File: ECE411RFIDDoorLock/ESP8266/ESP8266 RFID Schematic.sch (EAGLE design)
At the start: 32 parts, among them J4 1050170001, M1 SERVO, Q3 MMBT2222ALT1GOSCT-ND, T1 600mA/40V, T2 600mA/40V, U1 CP2104, U2 AP2112K-3.3TRG1, X1 ESP-12E

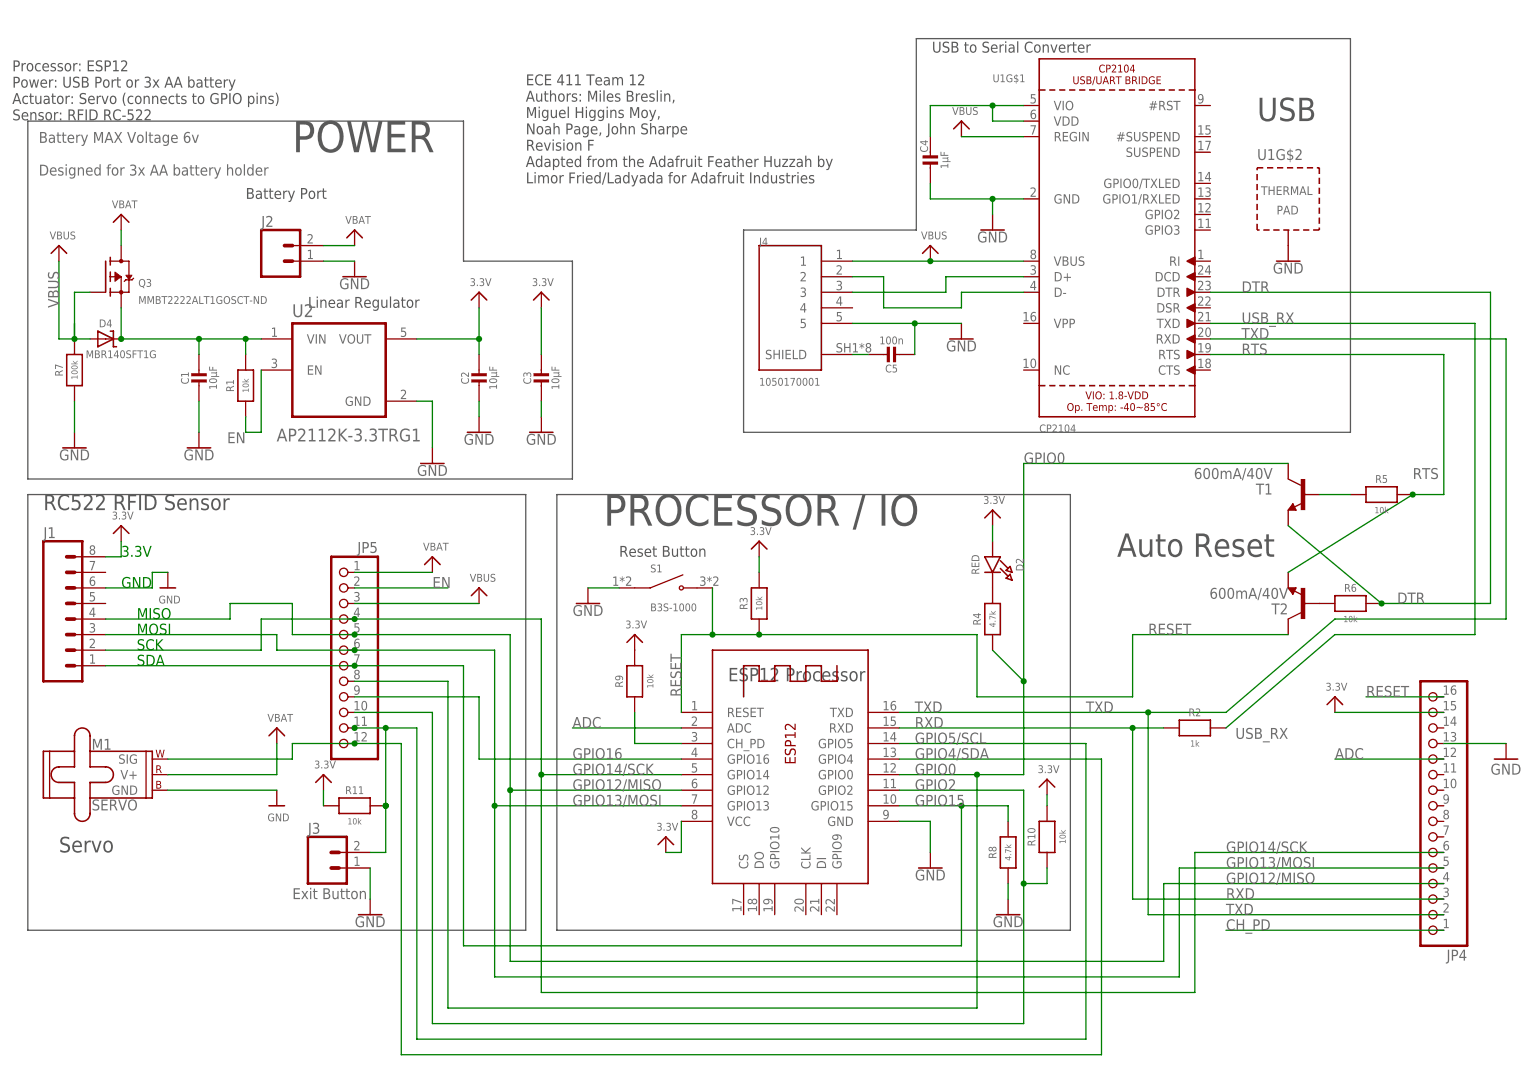
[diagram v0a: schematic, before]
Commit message: Revert
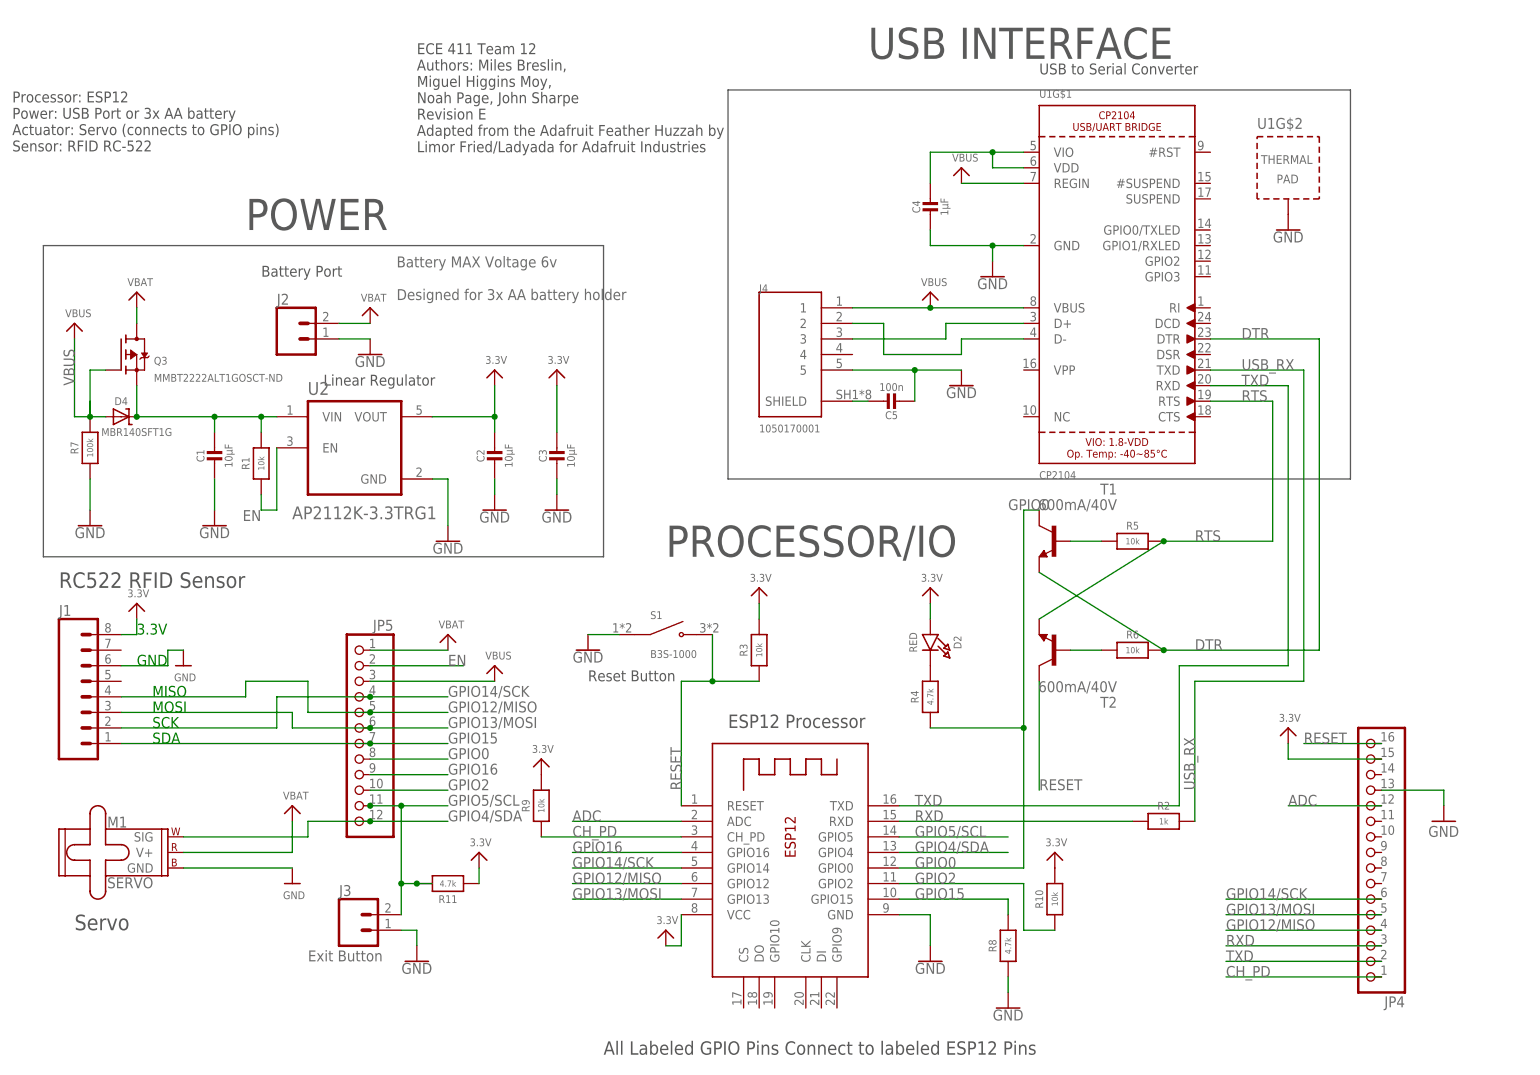
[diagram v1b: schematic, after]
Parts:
- R11: value 10k -> 4.7k
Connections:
- removed net N$4: R9.1, X1.CH_PD
- net CH_PD: now also R9.1, X1.CH_PD
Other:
- note added: "All Labeled GPIO Pins Connect to labeled ESP12 Pins"
- note added: "ECE 411 Team 12 Authors: Miles Breslin, Miguel Higgins Moy, Noah Page, John Sharpe Revision E Adapted from the Adafruit Feather Huzzah by Limor Fried/Ladyada for Adafruit Industries"
- note added: "PROCESSOR/IO"
- note added: "USB INTERFACE"
- note removed: "Auto Reset"
- note removed: "ECE 411 Team 12 Authors: Miles Breslin, Miguel Higgins Moy, Noah Page, John Sharpe Revision F Adapted from the Adafruit Feather Huzzah by Limor Fried/Ladyada for Adafruit Industries"
- note removed: "PROCESSOR / IO"
- note removed: "USB"
- moved on the sheet: C1, C2, C3, C4, C5, D2, D4, J1, J2, J3, J4, JP4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

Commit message: Readme update and organizing
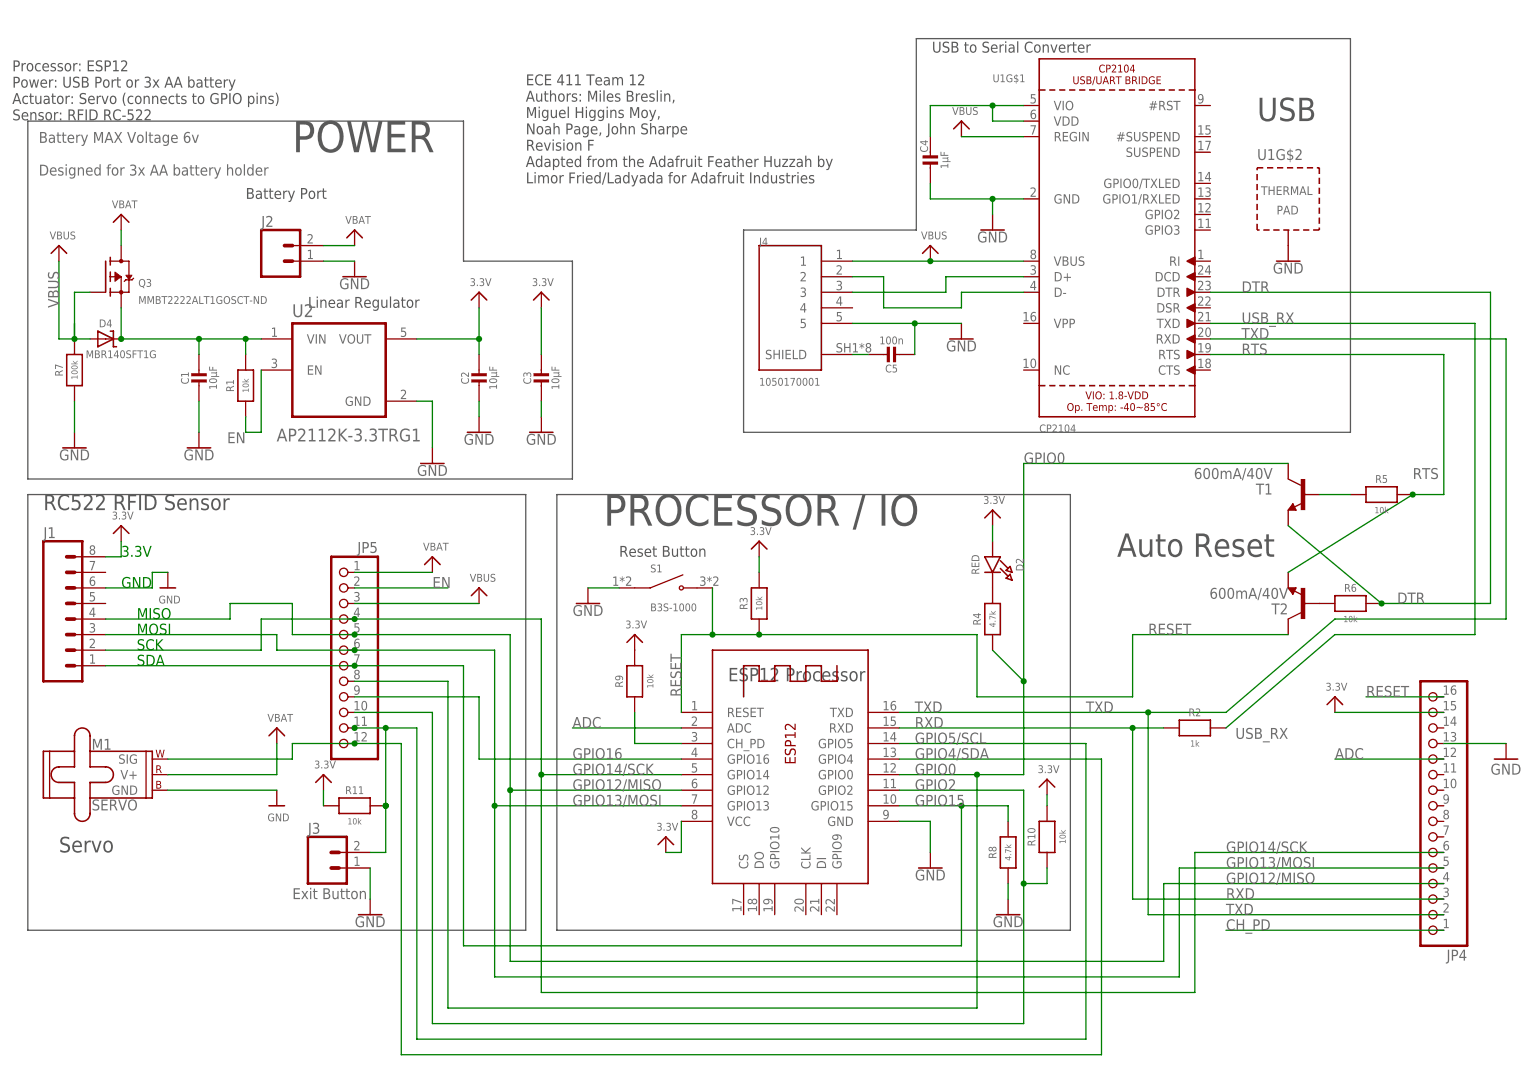
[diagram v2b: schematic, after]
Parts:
- R11: value 4.7k -> 10k
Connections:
- new net N$4: R9.1, X1.CH_PD
- net CH_PD: no longer R9.1, X1.CH_PD
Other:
- note added: "Auto Reset"
- note added: "ECE 411 Team 12 Authors: Miles Breslin, Miguel Higgins Moy, Noah Page, John Sharpe Revision F Adapted from the Adafruit Feather Huzzah by Limor Fried/Ladyada for Adafruit Industries"
- note added: "PROCESSOR / IO"
- note added: "USB"
- note removed: "All Labeled GPIO Pins Connect to labeled ESP12 Pins"
- note removed: "ECE 411 Team 12 Authors: Miles Breslin, Miguel Higgins Moy, Noah Page, John Sharpe Revision E Adapted from the Adafruit Feather Huzzah by Limor Fried/Ladyada for Adafruit Industries"
- note removed: "PROCESSOR/IO"
- note removed: "USB INTERFACE"
- moved on the sheet: C1, C2, C3, C4, C5, D2, D4, J1, J2, J3, J4, JP4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
